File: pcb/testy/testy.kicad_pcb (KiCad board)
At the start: 2 copper layers, 159 x 86 mm, 30 parts, among them SW0:0 SW_Push, SW0:1 SW_Push, SW0:2 SW_Push, SW1:0 SW_Push, SW1:1 SW_Push, SW1:2 SW_Push, U1 ProMicro

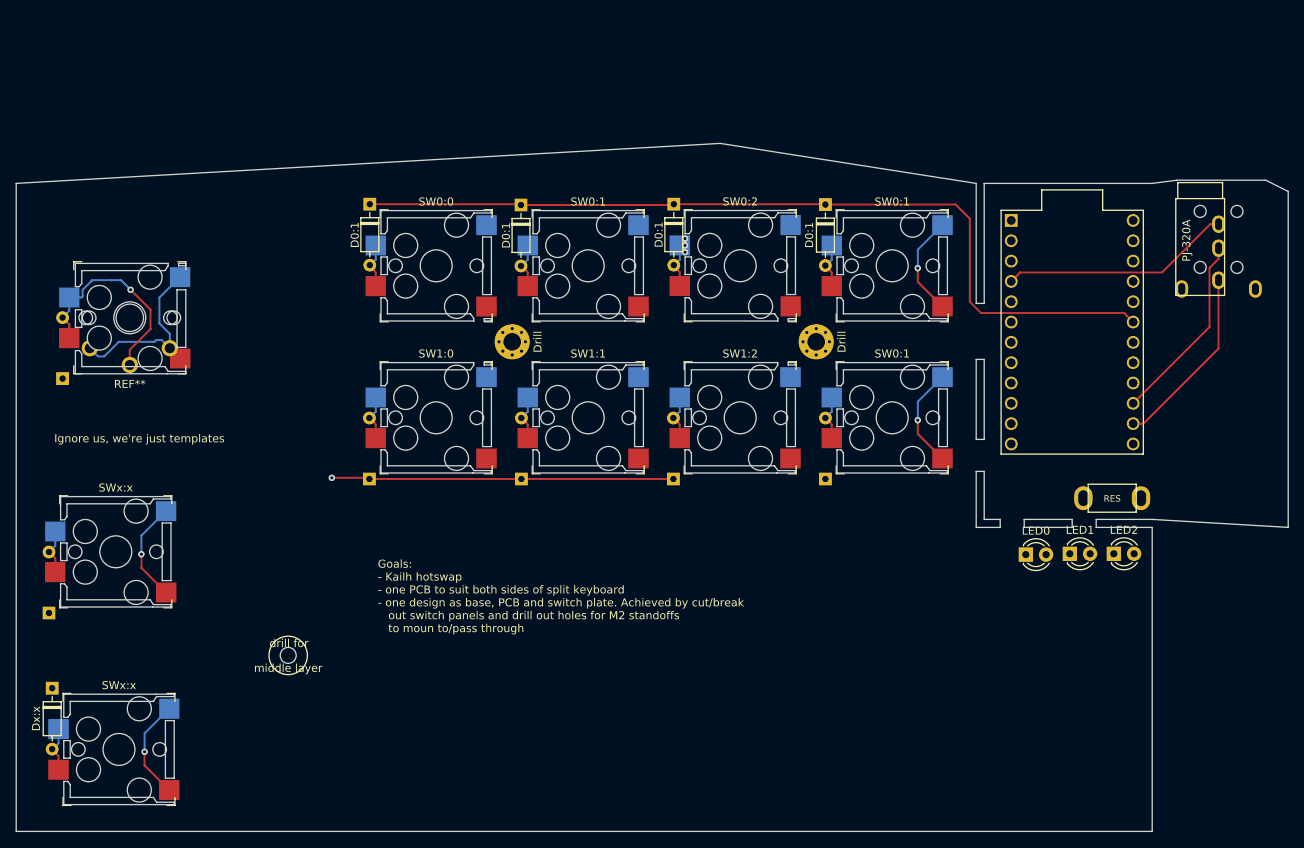
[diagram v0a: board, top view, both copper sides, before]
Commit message: feat: more playing with layout
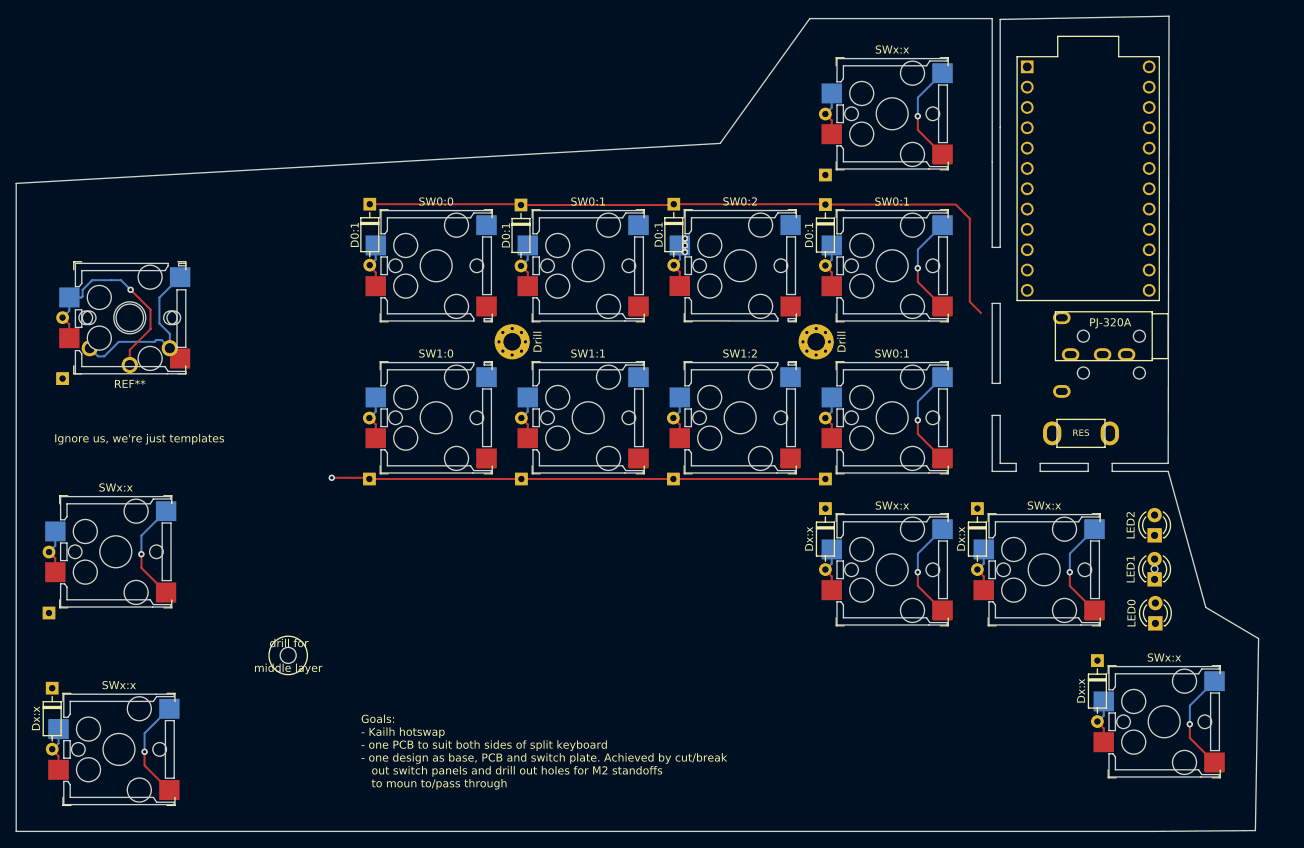
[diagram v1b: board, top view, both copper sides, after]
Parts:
- added Dx:x: 1N4148, Diode_THT:D_DO-35_SOD27_P7.62mm_Horizontal, B.Cu at (155.2, 41.0)
- added Dx:x: 1N4148, Diode_THT:D_DO-35_SOD27_P7.62mm_Horizontal, F.Cu at (189.2, 101.7)
- added Dx:x: 1N4148, Diode_THT:D_DO-35_SOD27_P7.62mm_Horizontal, F.Cu at (174.2, 82.7)
- added Dx:x: 1N4148, Diode_THT:D_DO-35_SOD27_P7.62mm_Horizontal, F.Cu at (155.2, 82.7)
- added SWx:x: SW_Push, footprints:Kailh_socket_reversible, F.Cu at (163.5, 33.3)
- added SWx:x: SW_Push, footprints:Kailh_socket_reversible, F.Cu at (197.5, 109.3)
- added SWx:x: SW_Push, footprints:Kailh_socket_reversible, F.Cu at (182.5, 90.3)
- added SWx:x: SW_Push, footprints:Kailh_socket_reversible, F.Cu at (163.5, 90.3)
- moved TRRS1 21.2 mm to (196.0, 63.4), turned to 270 degrees
- moved U1 19.3 mm to (188.0, 41.4)
- moved LED0 18.3 mm to (196.4, 97.0), turned to 90 degrees
- moved SW-reset1 12.2 mm to (187.1, 71.5), turned to 180 degrees
- moved LED1 11.1 mm to (196.3, 91.5), turned to 90 degrees
- moved LED2 5.59 mm to (196.3, 86.0), turned to 90 degrees
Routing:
- net (no net): track 87.7 -> 161.6 mm, vias 3 -> 7
- net VCC: track 28.9 -> 0.00 mm
- net GND: track 23.8 -> 0.00 mm
- net data: track 23.1 -> 0.00 mm
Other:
- board size 159 x 86 mm -> 155.3 x 101.9 mm
- board text added: "<--- Should we have centered holes to make drilling easier?"
